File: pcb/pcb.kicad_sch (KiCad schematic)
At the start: 94 parts, among them J1 N!N, J10 Conn_01x12_Socket, J11 Conn_01x12_Socket, J12 Conn_01x02_Socket, J2 Conn_01x12_Socket, J3 Conn_01x12_Socket, J4 Conn_01x12_Socket, J5 Conn_01x12_Socket, J6 Display_nice-view, J7 Conn_01x02_Socket, J8 Conn_01x12_Socket, J9 Conn_01x12_Socket, SW1 Switch, SW10 Switch, SW11 Switch, SW12 Switch, SW13 Switch, SW14 Switch, SW15 Switch, SW16 Switch, SW17 Switch, SW18 Switch, SW19 Switch, SW2 Switch, SW20 Switch, SW21 Switch, SW22 Switch, SW23 Switch, SW24 Switch, SW25 Switch, SW26 Switch, SW27 Switch, SW28 Switch, SW29 Switch, SW3 Switch, SW30 Switch, SW31 Switch, SW32 Switch, SW33 Switch, SW34 Switch, SW35 Switch, SW36 Switch, SW37 SW_Push, SW38 RotaryEncoder_Switch, SW4 Switch, SW5 Switch, SW6 Switch, SW7 Switch, SW8 Switch, SW9 Switch, U1 RollerEncoder_EVQWGD001

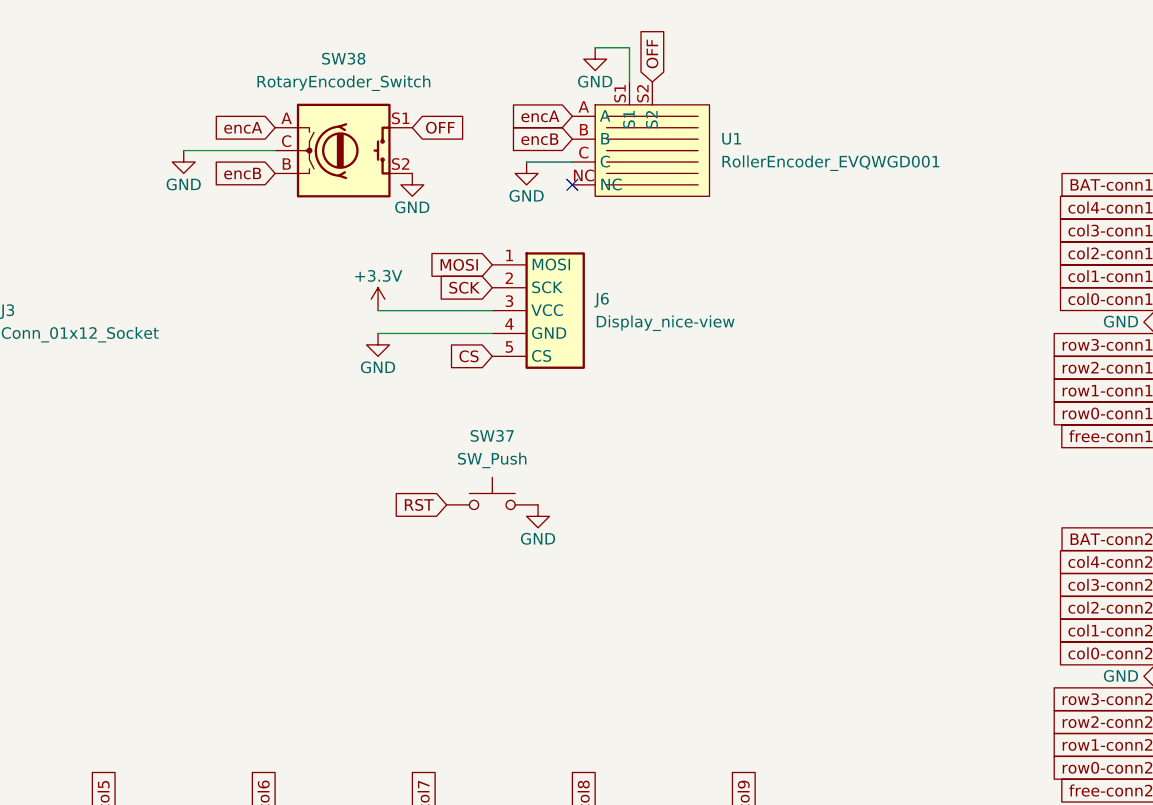
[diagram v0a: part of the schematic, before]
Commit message: update case and main pcb
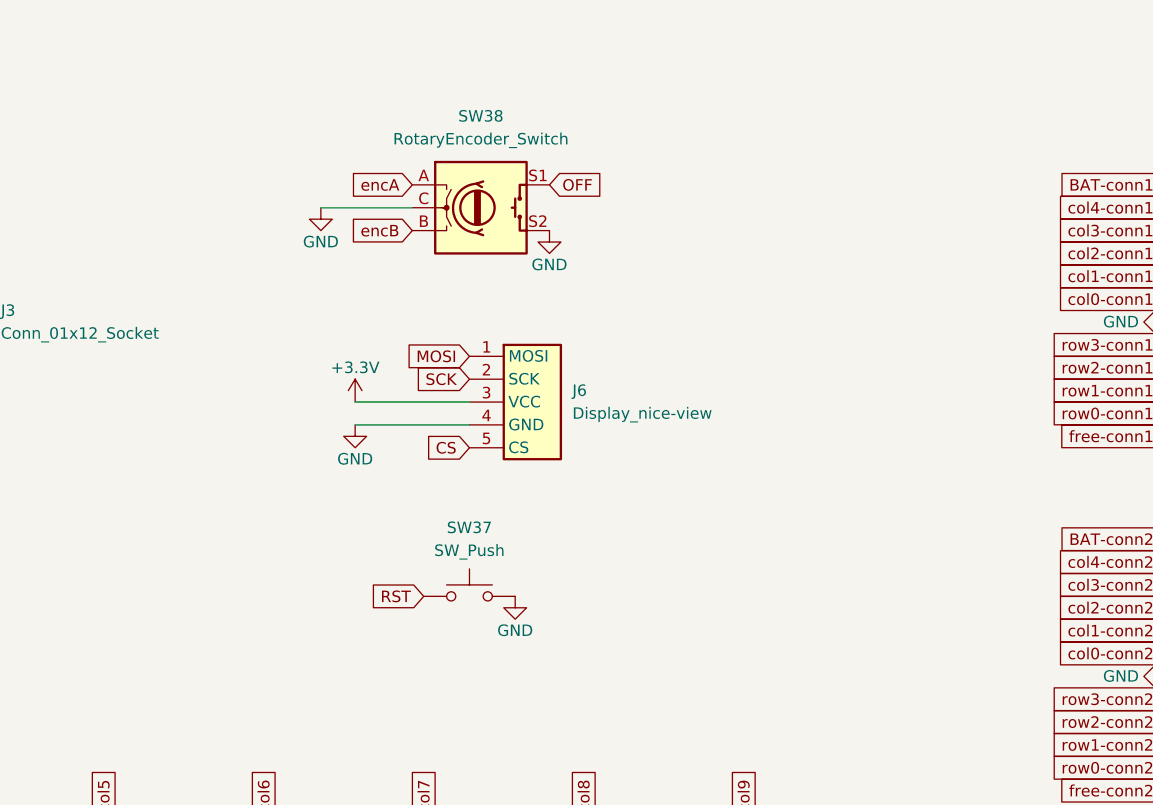
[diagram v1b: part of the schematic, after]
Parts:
- removed U1: RollerEncoder_EVQWGD001, zzkeeb:RotaryEncoder_EVQWGD001, symbol zzkeeb:RollerEncoder_EVQWGD001
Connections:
- no-connect marks 3 -> 2
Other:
- moved on the sheet: J6, SW37, SW38
